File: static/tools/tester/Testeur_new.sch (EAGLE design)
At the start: 35 parts, among them IC1 MEGA8-P, Q2 MFR475V

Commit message: [Tester] new design.
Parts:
- removed ALIM: (no value), pinhead:PINHD-1X2
- removed C1-CRYSTAL, C2-CRYSTAL: 20 pF, capacitor-wima:C5/5
- removed C1-REGULATOR, C1-REGULATOR1, C2-REGULATOR, C2-REGULATOR1: (no value), capacitor-wima:C5/5
- removed ENCODER-IHM: CI-11, piher:CI-11
- removed IC2, IC3: (no value), v-reg:78XXS
- removed JP1, JP2: (no value), pinhead:PINHD-2X12
- removed JP3: (no value), pinhead:PINHD-1X16
- removed Q1: (no value), special:XTAL/S
- removed R6: (no value), rcl:R-EU_0204/7
- removed SERVO-IHM, SERVO-IHM1, SERVO-IHM2: (no value), con-lstb:MA03-1
- removed SWITCH_5V: (no value), pinhead:PINHD-1X3
- removed X1: (no value), con-wago-500:W237-102
- added 0->3, 10->13, A0->A3: (no value), pinhead:PINHD-1X4
- added C1, C2: (no value), capacitor-wima:C5/3.5
- added ENCODER: CI-11, piher:CI-11
- added I²C: (no value), pinhead:PINHD-1X2
- added LCD: (no value), pinhead:PINHD-1X16
- added LCD_WIRES: (no value), pinhead:PINHD-1X6
- added PWM, SWITCH, SWITCH1: (no value), pinhead:PINHD-1X3
- added SERVO1, SERVO2: (no value), con-lstb:MA03-1
- added X2: (no value), con-wago-500:W237-102
- IC1: value MEGA8-P -> (none); device atmel:MEGA8-P -> v-reg:78XXS
- R3, R4: device resistor:R-EU_0204/7 -> rcl:R-EU_0204/7
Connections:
- removed net 5V_P/A: SERVO-IHM.2, SERVO-IHM1.2, SERVO-IHM2.2, SWITCH_5V.2
- removed net 5V_POW_IHM: JP2.3
- removed net ENCODER1: IC1.PD4(XCK/T0), JP1.24
- removed net ENCODER2: IC1.PD5(T1), JP1.23
- removed net GND_IHM: AR.1, C1-REGULATOR1.2, C2-REGULATOR1.2, CODER-IHM.2, ENCODER-IHMA.B, ENCODER-IHMB.D, I2C-IHM.2, IC3.GND, JP2.1, JP3.1, JP3.10, JP3.5, JP3.7, JP3.8, JP3.9, LED1.C, LED2.C, POTAR.3, Q2.E, RETURN_IHM.1, SERVO-IHM.1, SERVO-IHM1.1, SERVO-IHM2.1, X1-2.KL
- removed net INT_ODO1: IC1.PD2(INT0), JP1.18
- removed net LCD1: IC1.PD7(AIN1), JP1.19
- removed net LCD2: IC1.PB0(ICP), JP1.17
- removed net LCD3: IC1.PB1(OC1A), JP1.15
- removed net LCD5: IC1.PB4(MISO), JP1.9
- removed net LCD6: IC1.PB5(SCK), JP1.7
- removed net LED1: IC1.PC1(ADC1), R4.1
- removed net LED2: IC1.PC2(ADC2), R3.1
- removed net N$27: JP2.15, JP3.11
- removed net N$28: JP1.4, R4.2
- removed net N$29: JP2.13, JP3.12
- removed net N$30: JP2.9, JP3.13
- removed net N$34: JP2.7, JP3.14
- removed net N$35: JP2.11, R2.1, SERVO-IHM.3
- removed net N$36: JP2.8, RETURN_IHM.2
- removed net N$46: IC1.PC0(ADC0), R5.1, R6.2
- removed net N$7: JP1.6, R3.2
- removed net RETURN: IC1.PC3(ADC3), JP1.8
- removed net SCL: IC1.PC5(ADC5/SCL), JP1.12
- removed net SDA: IC1.PC4(ADC4/SDA), JP1.10
- removed net SELECT: IC1.PD6(AIN0), JP1.21
- removed net SENS_ODO: IC1.PD3(INT1), JP1.22
- removed net SERVO/PWM: IC1.PB3(MOSI/OC2), JP1.11
- removed net SERVO2: IC1.PD0(RXD), JP1.14
- removed net SERVO3: IC1.PD1(TXD), JP1.16
- removed net VCC: C2-REGULATOR.1, IC1.AVCC, IC1.VCC@1, IC2.OUT, JP1.5, R1.1
- removed net VCC_IHM: CODER-IHM.1, I2C-IHM.1, JP2.5, JP3.2, POTAR.2, SWITCH_5V.1
- new net 5V_ARDUINO: CODER-IHM.1, I2C-IHM.1, LCD.2, POTAR.2, SWITCH.3
- new net 5V_EXT: C2.1, IC1.OUT, SWITCH.1
- new net N$15: 10->13.3, PWM.3, R2.1
- new net N$24: AR.2, R4.2
- new net N$5: A0->A3.2, ENCODERA.C
- new net POWER: PWM.2, SERVO1.2, SERVO2.2, SWITCH1.2
- net 5V_POWER: now also SWITCH.2, SWITCH1.1; no longer C2-REGULATOR1.1, IC3.OUT, SWITCH_5V.3
- net ALIM_EXT: now also C1.1, IC1.IN, SWITCH1.3, X2-1.KL; no longer C1-REGULATOR1.1, IC3.IN, X1-1.KL
- net GND: now also AR.1, C1.2, C2.2, CODER-IHM.2, ENCODERA.B, ENCODERB.D, I2C-IHM.2, LCD.1, LCD.10, LCD.5, LCD.7, LCD.8, LCD.9, LED1.C, LED2.C, POTAR.3, PWM.1, Q2.E, R5.1, RETURN_IHM.1, SERVO1.1, SERVO2.1, X2-2.KL; no longer ALIM.1, C1-CRYSTAL.1, C1-REGULATOR.2, C2-CRYSTAL.1, C2-REGULATOR.2, IC1.GND@1, IC2.GND, JP1.1, R5.2
- net N$1: now also A0->A3.3, RETURN_IHM.2; no longer C1-CRYSTAL.2, IC1.PB6(XTAL1/TOSC1), Q1.1
- net N$10: now also I²C.2; no longer JP2.10
- net N$11: now also I²C.1; no longer JP2.12
- net N$12: now also R1.2; no longer JP2.4
- net N$13: now also 10->13.4, ENCODERB.E; no longer JP2.6, LED2.A
- net N$14: now also 0->3.4, SERVO1.3; no longer JP2.14, SERVO-IHM1.3
- net N$16: now also 0->3.2; no longer JP2.18
- net N$17: now also 0->3.1; no longer JP2.22
- net N$18: now also A0->A3.1, ENCODERA.A; no longer ENCODER-IHMA.A, JP2.24
- net N$2: now also LCD.11, LCD_WIRES.4; no longer C2-CRYSTAL.2, IC1.PB7(XTAL2/TOSC2), Q1.2
- net N$21: now also 10->13.2, R1.1; no longer ENCODER-IHMA.C, JP2.23
- net N$22: now also 10->13.1, R3.1; no longer ENCODER-IHMB.E, JP2.21
- net N$25: now also LCD.4, LCD_WIRES.6; no longer JP2.19, JP3.4
- net N$26: now also LCD.6, LCD_WIRES.5; no longer JP2.17, JP3.6
- net N$3: now also LCD.12, LCD_WIRES.3; no longer JP1.2, R6.1
- net N$37: now also A0->A3.4, R4.1, R5.2; no longer AR.2, JP2.2
- net N$39: now also LCD.3; no longer JP3.3
- net N$4: now also LCD.13, LCD_WIRES.2; no longer IC1.PC6(/RESET), R1.2
- net N$42: now also 0->3.3, SERVO2.3; no longer JP2.16, SERVO-IHM2.3
- net N$6: now also LCD.14, LCD_WIRES.1; no longer ALIM.2, C1-REGULATOR.1, IC2.IN
- net N$9: now also LED2.A, R3.2; no longer IC1.PB2(SS/OC1B), JP1.13

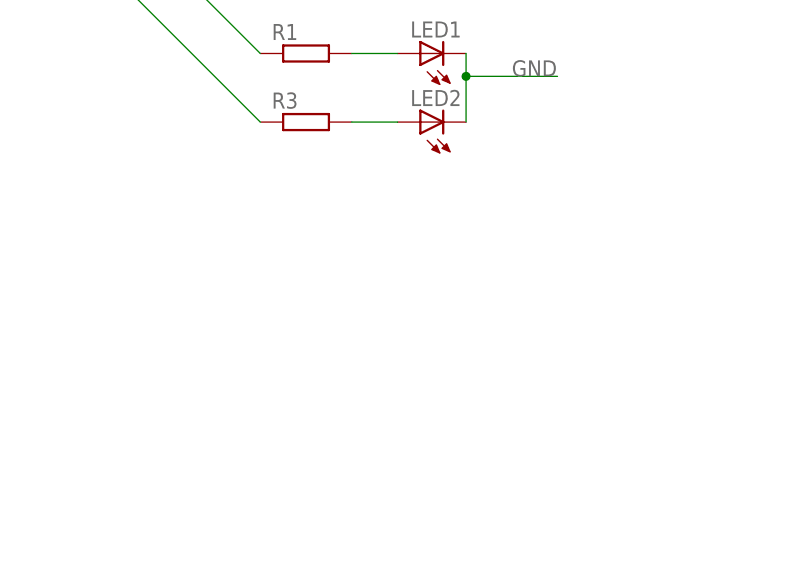
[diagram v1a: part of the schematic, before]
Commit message: [tester] continue new design.
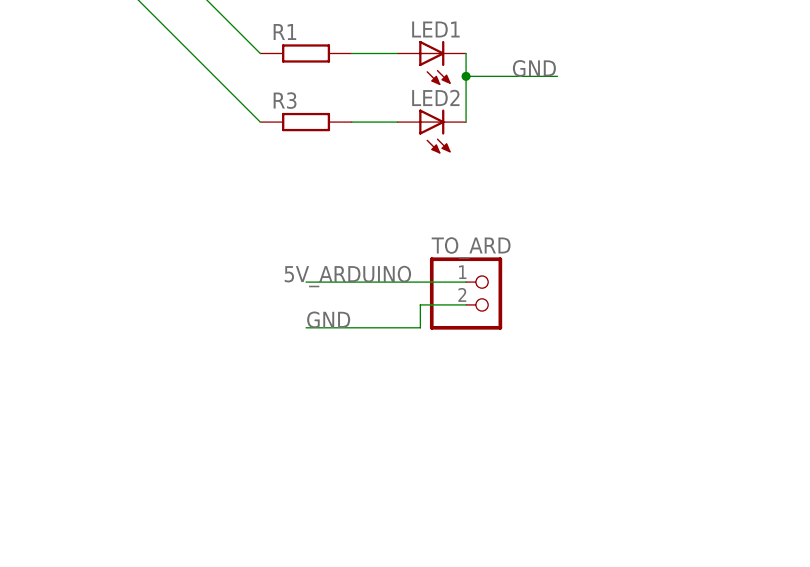
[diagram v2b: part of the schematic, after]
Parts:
- added TO_ARD: (no value), pinhead:PINHD-1X2
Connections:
- net 5V_ARDUINO: now also TO_ARD.1
- net GND: now also TO_ARD.2
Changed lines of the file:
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@@
 <part name="R5" library="rcl" deviceset="R-EU_" device="0204/7"/>
 <part name="SWITCH1" library="pinhead" deviceset="PINHD-1X3" device=""/>
+<part name="TO_ARD" library="pinhead" deviceset="PINHD-1X2" device=""/>
 </parts>
 <sheets>
@@
 <instance part="R5" gate="G$1" x="88.9" y="86.36" rot="R90"/>
 <instance part="SWITCH1" gate="A" x="-30.48" y="-22.86"/>
+<instance part="TO_ARD" gate="G$1" x="0" y="63.5"/>
 </instances>
 <busses>
@@
 <label x="88.9" y="78.74" size="1.778" layer="95"/>
 </segment>
+<segment>
+<pinref part="TO_ARD" gate="G$1" pin="2"/>
+<wire x1="-2.54" y1="63.5" x2="-7.62" y2="63.5" width="0.1524" layer="91"/>
+<wire x1="-7.62" y1="63.5" x2="-7.62" y2="60.96" width="0.1524" layer="91"/>
+<wire x1="-7.62" y1="60.96" x2="-20.32" y2="60.96" width="0.1524" layer="91"/>
+<label x="-20.32" y="60.96" size="1.778" layer="95"/>
+</segment>
 </net>
 <net name="N$10" class="0">
@@
 <label x="88.9" y="53.34" size="1.778" layer="95"/>
 </segment>
-</net>
+<segment>
+<pinref part="TO_ARD" gate="G$1" pin="1"/>
+<wire x1="-2.54" y1="66.04" x2="-20.32" y2="66.04" width="0.1524" layer="91"/>
+<label x="-22.86" y="66.04" size="1.778" layer="95"/>
+</segment>
+</net>
